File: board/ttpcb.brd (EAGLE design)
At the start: 72 x 72 mm, 9 parts

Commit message: u1
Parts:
- U$1, U$3, U$4, U$5, U$6, U$7, U$8, U$9: value QRE1113QRE1113GR-3D -> QRE1113QRE1113GR; device TinyTony_ShenzenReady:SOP180P460X170-4 -> TinyTony_ShenzenReady:QRE1113GR
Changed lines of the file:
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@@
 </autorouter>
 <elements>
-<element name="U$1" library="TinyTony_ShenzenReady" library_urn="urn:adsk.eagle:library:2159173" package="SOP180P460X170-4" package3d_urn="urn:adsk.eagle:package:4203844/1" value="QRE1113QRE1113GR-3D" x="0.08" y="4.9" smashed="yes">
+<element name="U$1" library="TinyTony_ShenzenReady" library_urn="urn:adsk.eagle:library:2159173" package="QRE1113GR" package3d_urn="urn:adsk.eagle:package:4203844/1" value="QRE1113QRE1113GR" x="0.08" y="4.9" smashed="yes">
 <attribute name="NAME" x="0.08" y="7.5336" size="1.27" layer="25" align="bottom-center"/>
 </element>
@@
 <attribute name="PROD_ID" value="IC-10828" x="14.59" y="7.32" size="1.778" layer="27" display="off"/>
 </element>
-<element name="U$3" library="TinyTony_ShenzenReady" library_urn="urn:adsk.eagle:library:2159173" package="SOP180P460X170-4" package3d_urn="urn:adsk.eagle:package:4203844/1" value="QRE1113QRE1113GR-3D" x="0.03" y="31.64" smashed="yes">
+<element name="U$3" library="TinyTony_ShenzenReady" library_urn="urn:adsk.eagle:library:2159173" package="QRE1113GR" package3d_urn="urn:adsk.eagle:package:4203844/1" value="QRE1113QRE1113GR" x="0.03" y="31.64" smashed="yes">
 <attribute name="NAME" x="0.03" y="34.2736" size="1.27" layer="25" align="bottom-center"/>
 </element>
-<element name="U$4" library="TinyTony_ShenzenReady" library_urn="urn:adsk.eagle:library:2159173" package="SOP180P460X170-4" package3d_urn="urn:adsk.eagle:package:4203844/1" value="QRE1113QRE1113GR-3D" x="0.06" y="8.73" smashed="yes">
+<element name="U$4" library="TinyTony_ShenzenReady" library_urn="urn:adsk.eagle:library:2159173" package="QRE1113GR" package3d_urn="urn:adsk.eagle:package:4203844/1" value="QRE1113QRE1113GR" x="0.06" y="8.73" smashed="yes">
 <attribute name="NAME" x="0.06" y="11.3636" size="1.27" layer="25" align="bottom-center"/>
 </element>
-<element name="U$5" library="TinyTony_ShenzenReady" library_urn="urn:adsk.eagle:library:2159173" package="SOP180P460X170-4" package3d_urn="urn:adsk.eagle:package:4203844/1" value="QRE1113QRE1113GR-3D" x="0.035" y="24.041" smashed="yes">
+<element name="U$5" library="TinyTony_ShenzenReady" library_urn="urn:adsk.eagle:library:2159173" package="QRE1113GR" package3d_urn="urn:adsk.eagle:package:4203844/1" value="QRE1113QRE1113GR" x="0.035" y="24.041" smashed="yes">
 <attribute name="NAME" x="0.035" y="26.6746" size="1.27" layer="25" align="bottom-center"/>
 </element>
-<element name="U$6" library="TinyTony_ShenzenReady" library_urn="urn:adsk.eagle:library:2159173" package="SOP180P460X170-4" package3d_urn="urn:adsk.eagle:package:4203844/1" value="QRE1113QRE1113GR-3D" x="0.035" y="27.817" smashed="yes">
+<element name="U$6" library="TinyTony_ShenzenReady" library_urn="urn:adsk.eagle:library:2159173" package="QRE1113GR" package3d_urn="urn:adsk.eagle:package:4203844/1" value="QRE1113QRE1113GR" x="0.035" y="27.817" smashed="yes">
 <attribute name="NAME" x="0.035" y="30.4506" size="1.27" layer="25" align="bottom-center"/>
 </element>
-<element name="U$7" library="TinyTony_ShenzenReady" library_urn="urn:adsk.eagle:library:2159173" package="SOP180P460X170-4" package3d_urn="urn:adsk.eagle:package:4203844/1" value="QRE1113QRE1113GR-3D" x="0.019" y="20.293" smashed="yes">
+<element name="U$7" library="TinyTony_ShenzenReady" library_urn="urn:adsk.eagle:library:2159173" package="QRE1113GR" package3d_urn="urn:adsk.eagle:package:4203844/1" value="QRE1113QRE1113GR" x="0.019" y="20.293" smashed="yes">
 <attribute name="NAME" x="0.019" y="22.9266" size="1.27" layer="25" align="bottom-center"/>
 </element>
-<element name="U$8" library="TinyTony_ShenzenReady" library_urn="urn:adsk.eagle:library:2159173" package="SOP180P460X170-4" package3d_urn="urn:adsk.eagle:package:4203844/1" value="QRE1113QRE1113GR-3D" x="0.035" y="16.419" smashed="yes">
+<element name="U$8" library="TinyTony_ShenzenReady" library_urn="urn:adsk.eagle:library:2159173" package="QRE1113GR" package3d_urn="urn:adsk.eagle:package:4203844/1" value="QRE1113QRE1113GR" x="0.035" y="16.419" smashed="yes">
 <attribute name="NAME" x="0.035" y="19.0526" size="1.27" layer="25" align="bottom-center"/>
 </element>
-<element name="U$9" library="TinyTony_ShenzenReady" library_urn="urn:adsk.eagle:library:2159173" package="SOP180P460X170-4" package3d_urn="urn:adsk.eagle:package:4203844/1" value="QRE1113QRE1113GR-3D" x="0.035" y="12.561" smashed="yes">
+<element name="U$9" library="TinyTony_ShenzenReady" library_urn="urn:adsk.eagle:library:2159173" package="QRE1113GR" package3d_urn="urn:adsk.eagle:package:4203844/1" value="QRE1113QRE1113GR" x="0.035" y="12.561" smashed="yes">
 <attribute name="NAME" x="0.035" y="15.1946" size="1.27" layer="25" align="bottom-center"/>
 </element>

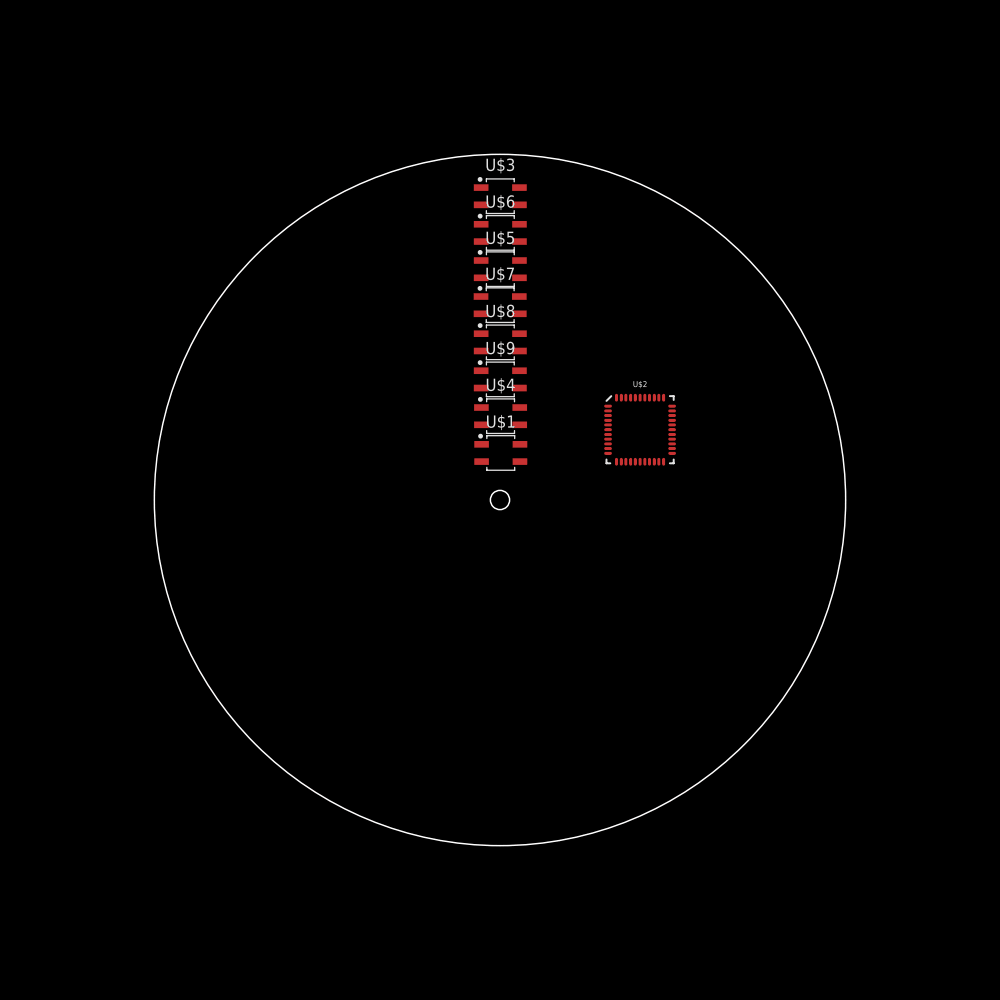
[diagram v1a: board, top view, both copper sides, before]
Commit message: svg
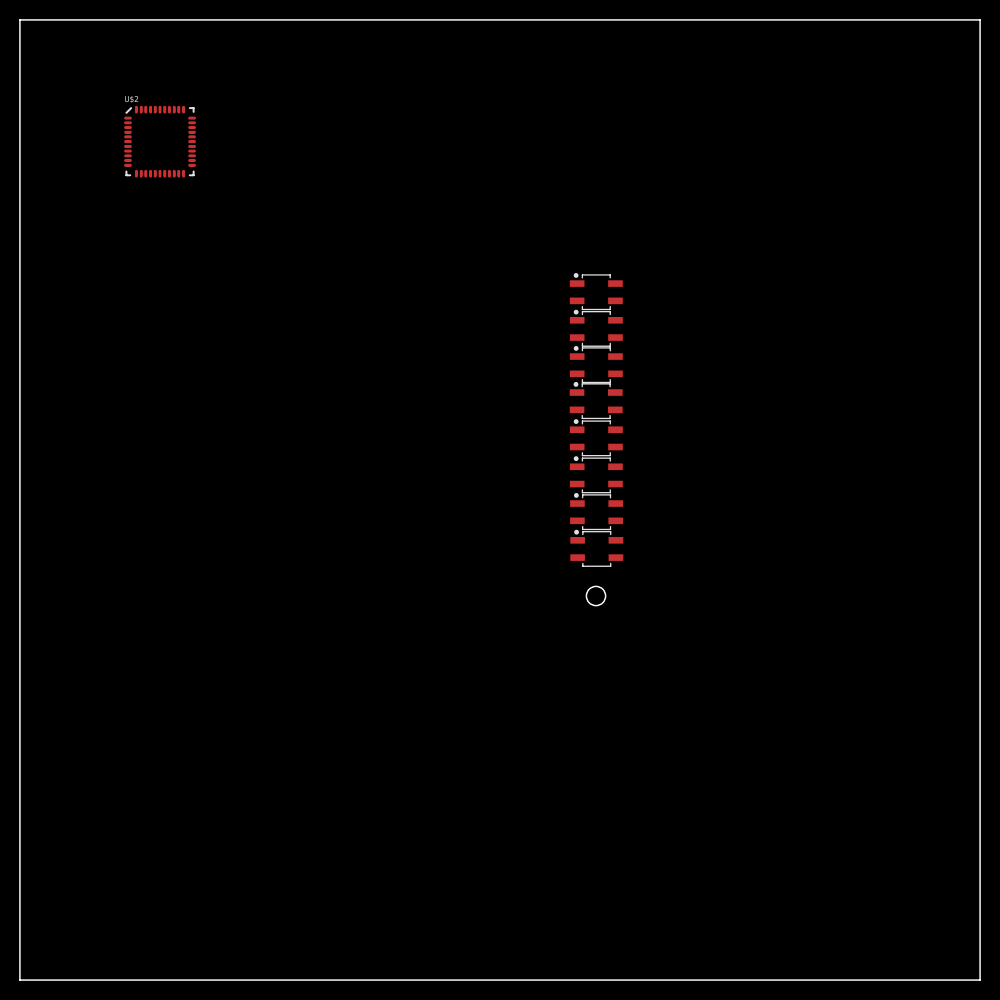
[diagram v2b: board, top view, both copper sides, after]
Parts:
- moved U$2 58.3 mm to (-35.4, 37.3)
- moved U$1 14.1 mm to (10.1, -5.10)
- moved U$3 14.1 mm to (10.0, 21.6)
- moved U$4 14.1 mm to (10.1, -1.27)
- moved U$5 14.1 mm to (10.0, 14.0)
- moved U$6 14.1 mm to (10.0, 17.8)
- moved U$7 14.1 mm to (10.0, 10.3)
- moved U$8 14.1 mm to (10.0, 6.42)
- moved U$9 14.1 mm to (10.0, 2.56)
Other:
- board size 72 x 72 mm -> 100 x 100 mm
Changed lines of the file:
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@@
 <board>
 <plain>
-<circle x="0" y="0" radius="36" width="0.1524" layer="20"/>
-<circle x="0" y="0" radius="1" width="0.1524" layer="20"/>
-<wire x1="-40" y1="40" x2="40" y2="40" width="0.1524" layer="51"/>
-<wire x1="40" y1="40" x2="40" y2="-40" width="0.1524" layer="51"/>
-<wire x1="40" y1="-40" x2="-40" y2="-40" width="0.1524" layer="51"/>
-<wire x1="-40" y1="-40" x2="-40" y2="40" width="0.1524" layer="51"/>
-<dimension x1="-40" y1="40" x2="40" y2="40" x3="0" y3="40" textsize="1.778" layer="51" dtype="horizontal"/>
-<dimension x1="0" y1="-36" x2="0" y2="36" x3="-50" y3="0" textsize="1.778" layer="51" dtype="diameter"/>
+<circle x="10" y="-10" radius="36" width="0.1524" layer="51"/>
+<circle x="10" y="-10" radius="1" width="0.1524" layer="20"/>
+<dimension x1="10" y1="-46" x2="10" y2="26" x3="-42.18" y3="-10" textsize="1.778" layer="51" dtype="diameter"/>
+<wire x1="50" y1="-50" x2="50" y2="50" width="0.1524" layer="20"/>
+<wire x1="50" y1="50" x2="-50" y2="50" width="0.1524" layer="20"/>
+<wire x1="-50" y1="50" x2="-50" y2="-50" width="0.1524" layer="20"/>
+<wire x1="-50" y1="-50" x2="50" y2="-50" width="0.1524" layer="20"/>
+<dimension x1="-50" y1="50" x2="-50" y2="-50" x3="-51.88" y3="0" textsize="1.778" layer="20"/>
 </plain>
 <attributes>
@@
 </autorouter>
 <elements>
-<element name="U$1" library="TinyTony_ShenzenReady" library_urn="urn:adsk.eagle:library:2159173" package="QRE1113GR" package3d_urn="urn:adsk.eagle:package:4203844/1" value="QRE1113QRE1113GR" x="0.08" y="4.9" smashed="yes">
-<attribute name="NAME" x="0.08" y="7.5336" size="1.27" layer="25" align="bottom-center"/>
+<element name="U$1" library="TinyTony_ShenzenReady" library_urn="urn:adsk.eagle:library:2159173" package="QRE1113GR" package3d_urn="urn:adsk.eagle:package:4203844/1" value="QRE1113QRE1113GR" x="10.08" y="-5.1" smashed="yes"/>
+<element name="U$2" library="SparkFun-IC-Microcontroller" library_urn="urn:adsk.eagle:library:525" package="QFN-44-NOPAD_1:1" package3d_urn="urn:adsk.eagle:package:38952/1" value="32U4" x="-35.41" y="37.32" smashed="yes">
+<attribute name="NAME" x="-38.37" y="41.455" size="0.6096" layer="25" font="vector" ratio="20" align="bottom-center"/>
+<attribute name="PROD_ID" value="IC-10828" x="-35.41" y="37.32" size="1.778" layer="27" display="off"/>
+<attribute name="VALUE" x="-33.22" y="31.96" size="1.016" layer="27" font="vector" ratio="20" align="bottom-center"/>
 </element>
-<element name="U$2" library="SparkFun-IC-Microcontroller" library_urn="urn:adsk.eagle:library:525" package="QFN-44-NOPAD_1:1" package3d_urn="urn:adsk.eagle:package:38952/1" value="32U4" x="14.59" y="7.32">
-<attribute name="PROD_ID" value="IC-10828" x="14.59" y="7.32" size="1.778" layer="27" display="off"/>
-</element>
-<element name="U$3" library="TinyTony_ShenzenReady" library_urn="urn:adsk.eagle:library:2159173" package="QRE1113GR" package3d_urn="urn:adsk.eagle:package:4203844/1" value="QRE1113QRE1113GR" x="0.03" y="31.64" smashed="yes">
-<attribute name="NAME" x="0.03" y="34.2736" size="1.27" layer="25" align="bottom-center"/>
-</element>
-<element name="U$4" library="TinyTony_ShenzenReady" library_urn="urn:adsk.eagle:library:2159173" package="QRE1113GR" package3d_urn="urn:adsk.eagle:package:4203844/1" value="QRE1113QRE1113GR" x="0.06" y="8.73" smashed="yes">
-<attribute name="NAME" x="0.06" y="11.3636" size="1.27" layer="25" align="bottom-center"/>
-</element>
-<element name="U$5" library="TinyTony_ShenzenReady" library_urn="urn:adsk.eagle:library:2159173" package="QRE1113GR" package3d_urn="urn:adsk.eagle:package:4203844/1" value="QRE1113QRE1113GR" x="0.035" y="24.041" smashed="yes">
-<attribute name="NAME" x="0.035" y="26.6746" size="1.27" layer="25" align="bottom-center"/>
-</element>
-<element name="U$6" library="TinyTony_ShenzenReady" library_urn="urn:adsk.eagle:library:2159173" package="QRE1113GR" package3d_urn="urn:adsk.eagle:package:4203844/1" value="QRE1113QRE1113GR" x="0.035" y="27.817" smashed="yes">
-<attribute name="NAME" x="0.035" y="30.4506" size="1.27" layer="25" align="bottom-center"/>
-</element>
-<element name="U$7" library="TinyTony_ShenzenReady" library_urn="urn:adsk.eagle:library:2159173" package="QRE1113GR" package3d_urn="urn:adsk.eagle:package:4203844/1" value="QRE1113QRE1113GR" x="0.019" y="20.293" smashed="yes">
-<attribute name="NAME" x="0.019" y="22.9266" size="1.27" layer="25" align="bottom-center"/>
-</element>
-<element name="U$8" library="TinyTony_ShenzenReady" library_urn="urn:adsk.eagle:library:2159173" package="QRE1113GR" package3d_urn="urn:adsk.eagle:package:4203844/1" value="QRE1113QRE1113GR" x="0.035" y="16.419" smashed="yes">
-<attribute name="NAME" x="0.035" y="19.0526" size="1.27" layer="25" align="bottom-center"/>
-</element>
-<element name="U$9" library="TinyTony_ShenzenReady" library_urn="urn:adsk.eagle:library:2159173" package="QRE1113GR" package3d_urn="urn:adsk.eagle:package:4203844/1" value="QRE1113QRE1113GR" x="0.035" y="12.561" smashed="yes">
-<attribute name="NAME" x="0.035" y="15.1946" size="1.27" layer="25" align="bottom-center"/>
-</element>
+<element name="U$3" library="TinyTony_ShenzenReady" library_urn="urn:adsk.eagle:library:2159173" package="QRE1113GR" package3d_urn="urn:adsk.eagle:package:4203844/1" value="QRE1113QRE1113GR" x="10.03" y="21.64" smashed="yes"/>
+<element name="U$4" library="TinyTony_ShenzenReady" library_urn="urn:adsk.eagle:library:2159173" package="QRE1113GR" package3d_urn="urn:adsk.eagle:package:4203844/1" value="QRE1113QRE1113GR" x="10.06" y="-1.27" smashed="yes"/>
+<element name="U$5" library="TinyTony_ShenzenReady" library_urn="urn:adsk.eagle:library:2159173" package="QRE1113GR" package3d_urn="urn:adsk.eagle:package:4203844/1" value="QRE1113QRE1113GR" x="10.035" y="14.041" smashed="yes"/>
+<element name="U$6" library="TinyTony_ShenzenReady" library_urn="urn:adsk.eagle:library:2159173" package="QRE1113GR" package3d_urn="urn:adsk.eagle:package:4203844/1" value="QRE1113QRE1113GR" x="10.035" y="17.817" smashed="yes"/>
+<element name="U$7" library="TinyTony_ShenzenReady" library_urn="urn:adsk.eagle:library:2159173" package="QRE1113GR" package3d_urn="urn:adsk.eagle:package:4203844/1" value="QRE1113QRE1113GR" x="10.019" y="10.293" smashed="yes"/>
+<element name="U$8" library="TinyTony_ShenzenReady" library_urn="urn:adsk.eagle:library:2159173" package="QRE1113GR" package3d_urn="urn:adsk.eagle:package:4203844/1" value="QRE1113QRE1113GR" x="10.035" y="6.419" smashed="yes"/>
+<element name="U$9" library="TinyTony_ShenzenReady" library_urn="urn:adsk.eagle:library:2159173" package="QRE1113GR" package3d_urn="urn:adsk.eagle:package:4203844/1" value="QRE1113QRE1113GR" x="10.035" y="2.561" smashed="yes"/>
 </elements>
 <signals>
